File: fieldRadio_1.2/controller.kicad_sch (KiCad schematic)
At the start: 55 parts, among them J11 Conn_01x04, Q19 BSS138, U31 MIC5235-3.3YM5, Y1 32.768kHz

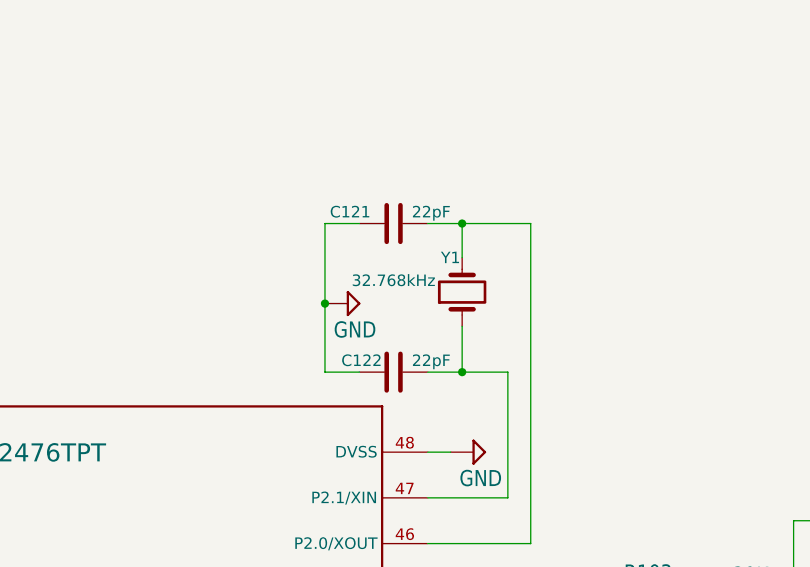
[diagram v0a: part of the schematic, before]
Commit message: continued symbol property updates
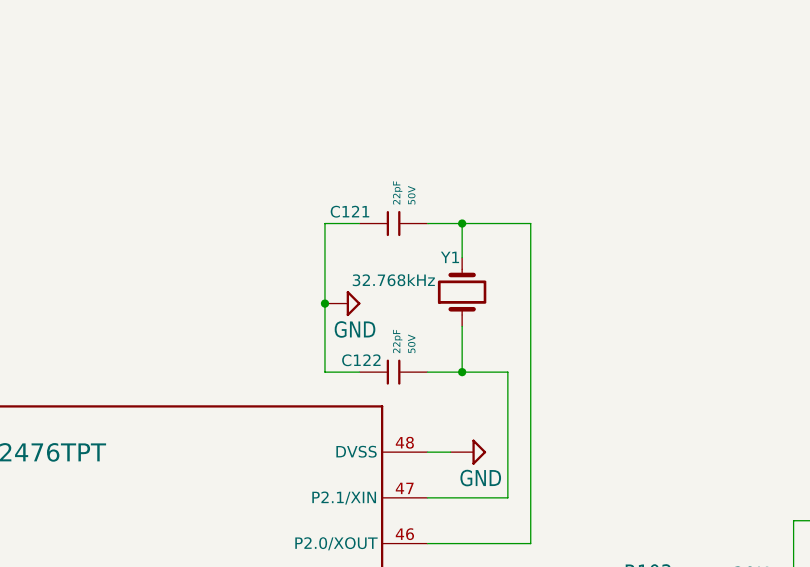
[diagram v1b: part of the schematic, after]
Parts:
- C105, C107, C109, C110, C111, C112, C113, C117, C129, C130, C131, C132, C136, C140: JLCPCB (none) -> C14663
- C106, C108: JLCPCB (none) -> C15849
- C114: JLCPCB (none) -> C15850
- C120: JLCPCB (none) -> C1588
- C121, C122: footprint Capacitor_SMD:C_0603_1608Metric_Pad1.08x0.95mm_HandSolder -> PCM_JLCPCB:C_0603; symbol Device:C -> PCM_JLCPCB-Capacitors:0603,22pF; Attrition Qty (none) -> 10; Capacitance (none) -> 22pF; Category (none) -> Capacitors,Multilayer Ceramic Capacitors MLCC - SMD/SMT; Class (none) -> Basic Component; JLCPCB (none) -> C1653; LCSC (none) -> C1653; Manufacturer (none) -> Samsung Electro-Mechanics; Minimum Qty (none) -> 20; Part (none) -> CL10C220JB8NNNC; Price (none) -> 0.007USD; Process (none) -> SMT; Stock (none) -> 1531147; Temperature Coefficient (none) -> C0G; Tolerance (none) -> ±5%; Voltage Rated (none) -> 50V
- J11, RV2: now left out of the parts list
- Q19: JLCPCB (none) -> C7420339
- R100, R101, R102, R107, R108, R116, R118, R124, R90, R95, R97, R99: JLCPCB (none) -> C21190
- R103, R104, R105, R106, R115, R117, R119, R92, R94, R96, R98: JLCPCB (none) -> C23153
- R110, R111: JLCPCB (none) -> C13167
- R112: JLCPCB (none) -> C25819
- R89: JLCPCB (none) -> C23260
- R91: JLCPCB (none) -> C23138
- R93: JLCPCB (none) -> C22775
- U31: JLCPCB (none) -> C7202997
